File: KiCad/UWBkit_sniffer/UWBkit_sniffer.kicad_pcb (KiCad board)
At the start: 4 copper layers, 85.4 x 59.7 mm, 74 parts, among them J1 Conn_Coaxial, J10 Conn_SPIM, J2 Conn_SWD, J3 Conn_GPIO, J4 Conn_01x04, J5 Conn_I2C2, J6 USB_C_Receptacle_USB2.0_14P, J7 USB_C_Receptacle_USB2.0_14P, J8 Conn_SPIS, J9 Conn_I2C1, SW1 SW_Push, SW2 SW_Slide_DPDT, U1 LBUA5QJ2AB, U2 CP2104, U4 XC9285B33CMR-G, U5 IP4234CZ6, U6 IP4234CZ6

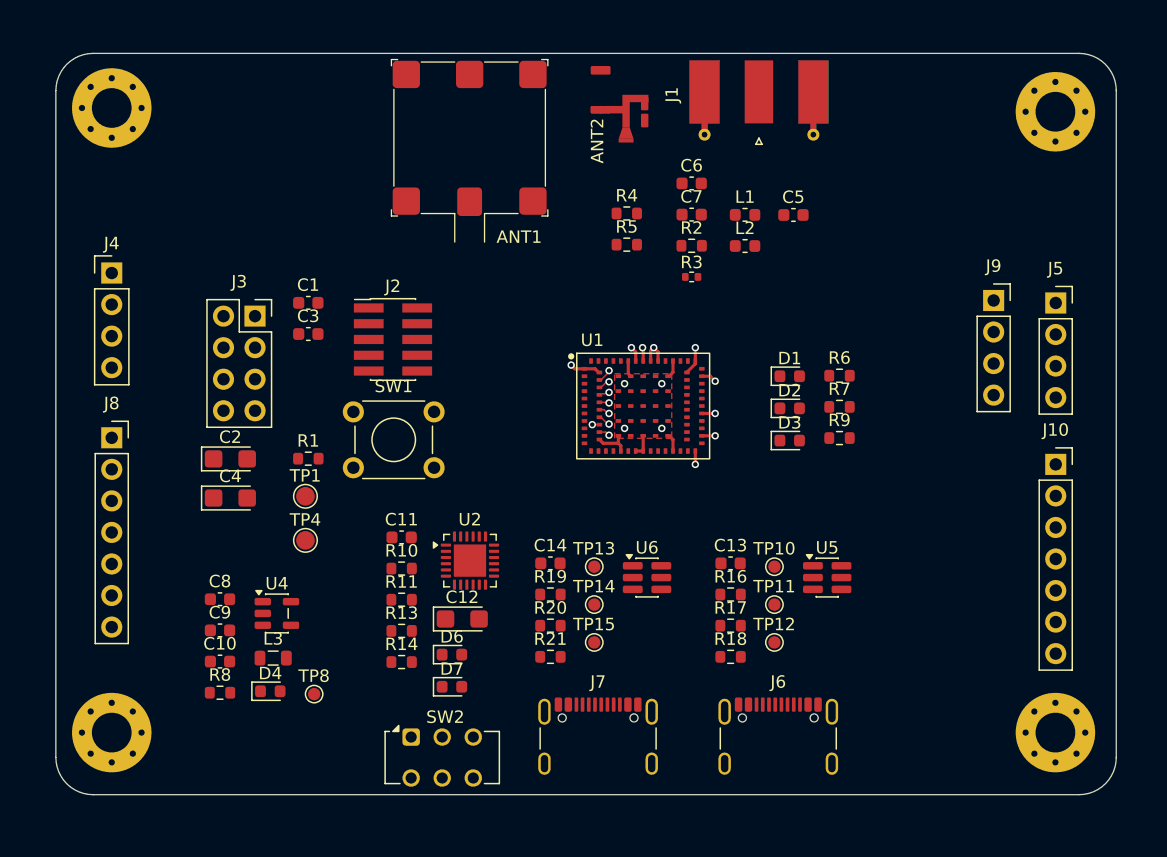
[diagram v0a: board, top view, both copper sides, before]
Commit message: First version of PCB
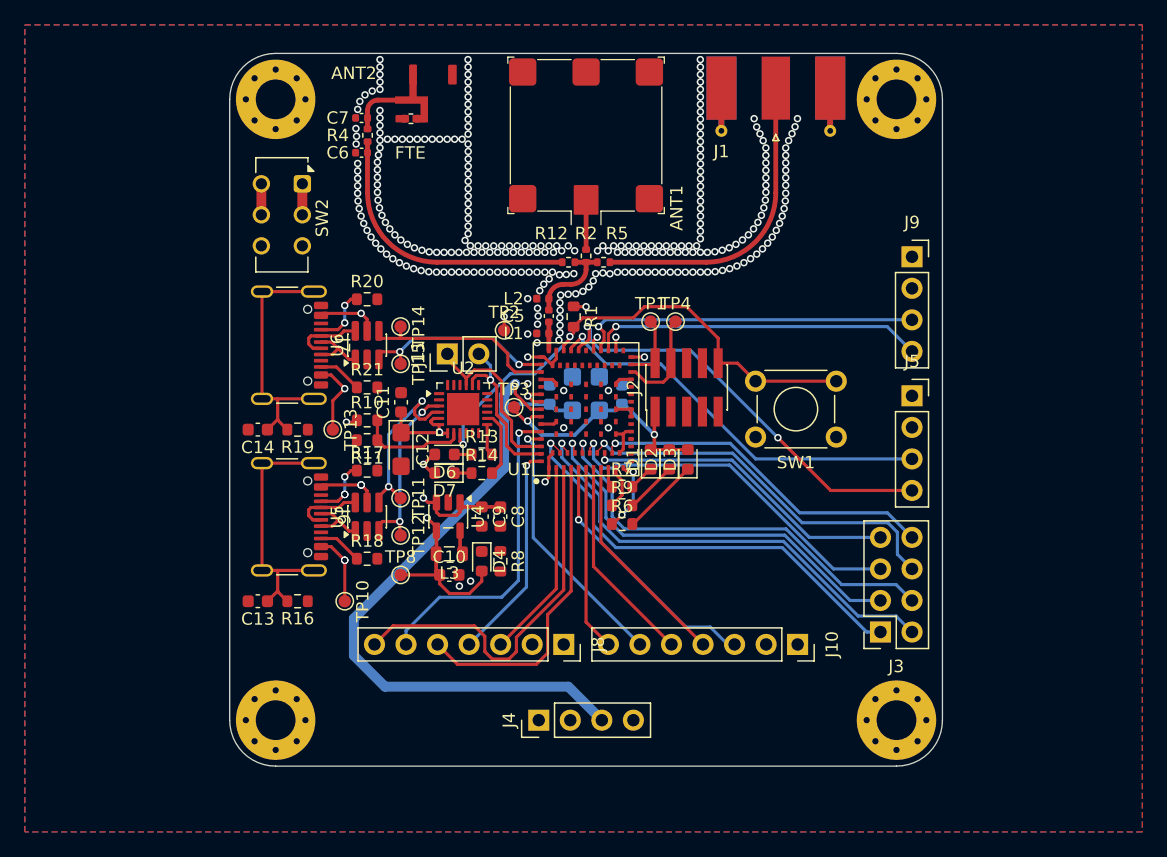
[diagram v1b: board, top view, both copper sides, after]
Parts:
- added J11: Conn_01x02, Connector_PinHeader_2.54mm:PinHeader_1x02_P2.54mm_Vertical, F.Cu at (149.4, 80.2)
- added R12: 0R, Resistor_SMD:R_0402_1005Metric, F.Cu at (159.2, 72.8)
- added TP2: TestPoint_Small, TestPoint:TestPoint_Pad_D1.0mm, F.Cu at (154.0, 78.3)
- added TP3: TestPoint_Small, TestPoint:TestPoint_Pad_D1.0mm, F.Cu at (154.8, 84.5)
- C1, C2, C3, C4: moved to B.Cu
- C5, C6, C7: footprint Capacitor_SMD:C_0603_1608Metric -> Capacitor_SMD:C_0402_1005Metric
- L1, L2: footprint Inductor_SMD:L_0603_1608Metric -> Inductor_SMD:L_0402_1005Metric
- R2, R4, R5: footprint Resistor_SMD:R_0603_1608Metric -> Resistor_SMD:R_0402_1005Metric
- TP1, TP4: footprint TestPoint:TestPoint_Pad_D1.5mm -> TestPoint:TestPoint_Pad_D1.0mm
- moved J3 56.4 mm to (184.3, 102.6), turned to 180 degrees
- moved J4 49.8 mm to (156.8, 109.7), turned to 90 degrees
- moved SW2 45.4 mm to (137.8, 66.5), turned to -90 degrees
- moved J6 44.7 mm to (135.6, 93.3), turned to -90 degrees
- moved J7 41.7 mm to (135.6, 79.5), turned to -90 degrees
- moved J8 40.0 mm to (158.8, 103.6), turned to -90 degrees
- moved SW1 38.9 mm to (180.8, 86.9), turned to 180 degrees
- moved C13 38.2 mm to (134.2, 100.1), turned to 180 degrees
- moved U5 37.4 mm to (143.0, 93.3), turned to 90 degrees
- moved R16 34.9 mm to (137.4, 100.1)
- moved TP10 34.7 mm to (141.2, 100.1), turned to -90 degrees
- moved TP4 34.6 mm to (167.8, 77.6)
- moved R17 31.8 mm to (143.0, 89.6)
- moved TP12 31.3 mm to (145.7, 94.8), turned to -90 degrees
- moved TP11 31.3 mm to (145.7, 91.8), turned to -90 degrees
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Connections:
- C6 pad 1: /CPU/ANT1 -> Net-(C6-Pad1)
- R14 pad 1: Net-(U2-TXT/GPIO.0) -> Net-(D7-K)
- R14 pad 2: Net-(D7-K) -> Net-(U2-TXT/GPIO.0)
- R2 pad 2: Net-(ANT2-Pad1) -> Net-(ANT1-Pad1)
- R4 pad 1: /CPU/ANT1 -> Net-(C6-Pad1)
- R4 pad 2: Net-(J1-In) -> Net-(ANT2-Pad1)
- R5 pad 2: Net-(ANT1-Pad1) -> Net-(J1-In)
- R6 pad 1: Net-(D3-K) -> /CPU/LED3
- R6 pad 2: /CPU/LED3 -> Net-(D3-K)
- SW2 pad 1: /USB-C_Connector_1/VBUS -> /USB-C_Connector_2/VBUS
- SW2 pad 2: /USB-C_Connector_1/VBUS -> /USB-C_Connector_2/VBUS
- SW2 pad 3: +5V -> SOC_VBUS
- SW2 pad 4: SOC_VBUS -> +5V
- SW2 pad 5: /USB-C_Connector_2/VBUS -> /USB-C_Connector_1/VBUS
- SW2 pad 6: /USB-C_Connector_2/VBUS -> /USB-C_Connector_1/VBUS
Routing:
- net +3V3: track 3.62 -> 156.0 mm, vias 2 -> 7
- net SOC_VBUS: track 1.10 -> 84.5 mm, vias 1 -> 2
- net +5V: track 0.00 -> 73.2 mm, vias 0 -> 2
- net /USB-C_Connector_1/VBUS: track 0.00 -> 51.2 mm, vias 0 -> 4
- net /nRST: track 0.00 -> 42.1 mm, vias 0 -> 7
- net Net-(J3-Pin_2): track 0.96 -> 37.4 mm
- net Net-(J3-Pin_1): track 1.14 -> 35.8 mm
- net /CPU/I2C2_SDA: track 0.00 -> 34.5 mm, vias 0 -> 2
- net Net-(J3-Pin_4): track 0.80 -> 34.6 mm
- net /USB-C_Connector_2/VBUS: track 0.00 -> 33.1 mm, vias 0 -> 2
- net /CPU/I2C2_SCL: track 0.00 -> 32.3 mm, vias 0 -> 1
- net Net-(J3-Pin_3): track 0.86 -> 32.8 mm
- net /CPU/SPIS_CS: track 0.00 -> 30.5 mm
- net Net-(J3-Pin_6): track 1.00 -> 31.0 mm
- net Net-(J3-Pin_5): track 0.90 -> 29.1 mm
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- added copper zone on B.Cu, net GND
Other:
- board size 85.4 x 59.7 mm -> 57.4 x 57.4 mm
- board text added: "FTE"
